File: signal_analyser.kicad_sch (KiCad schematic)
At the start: 0 parts

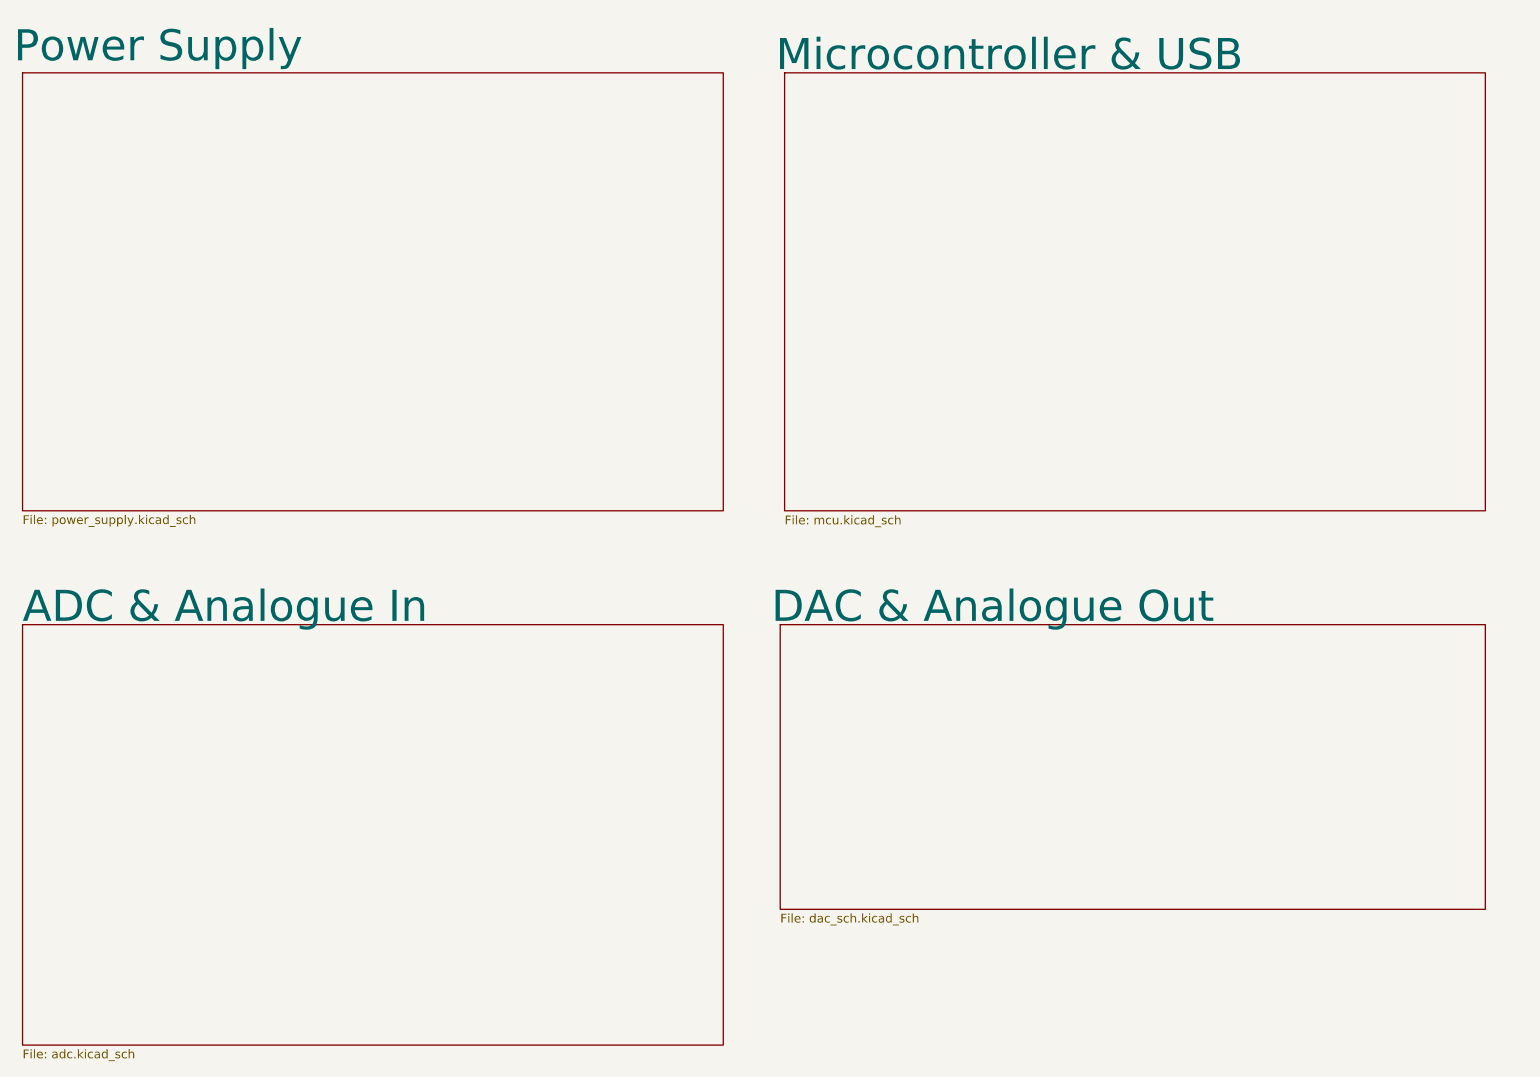
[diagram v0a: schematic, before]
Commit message: ERC valid.
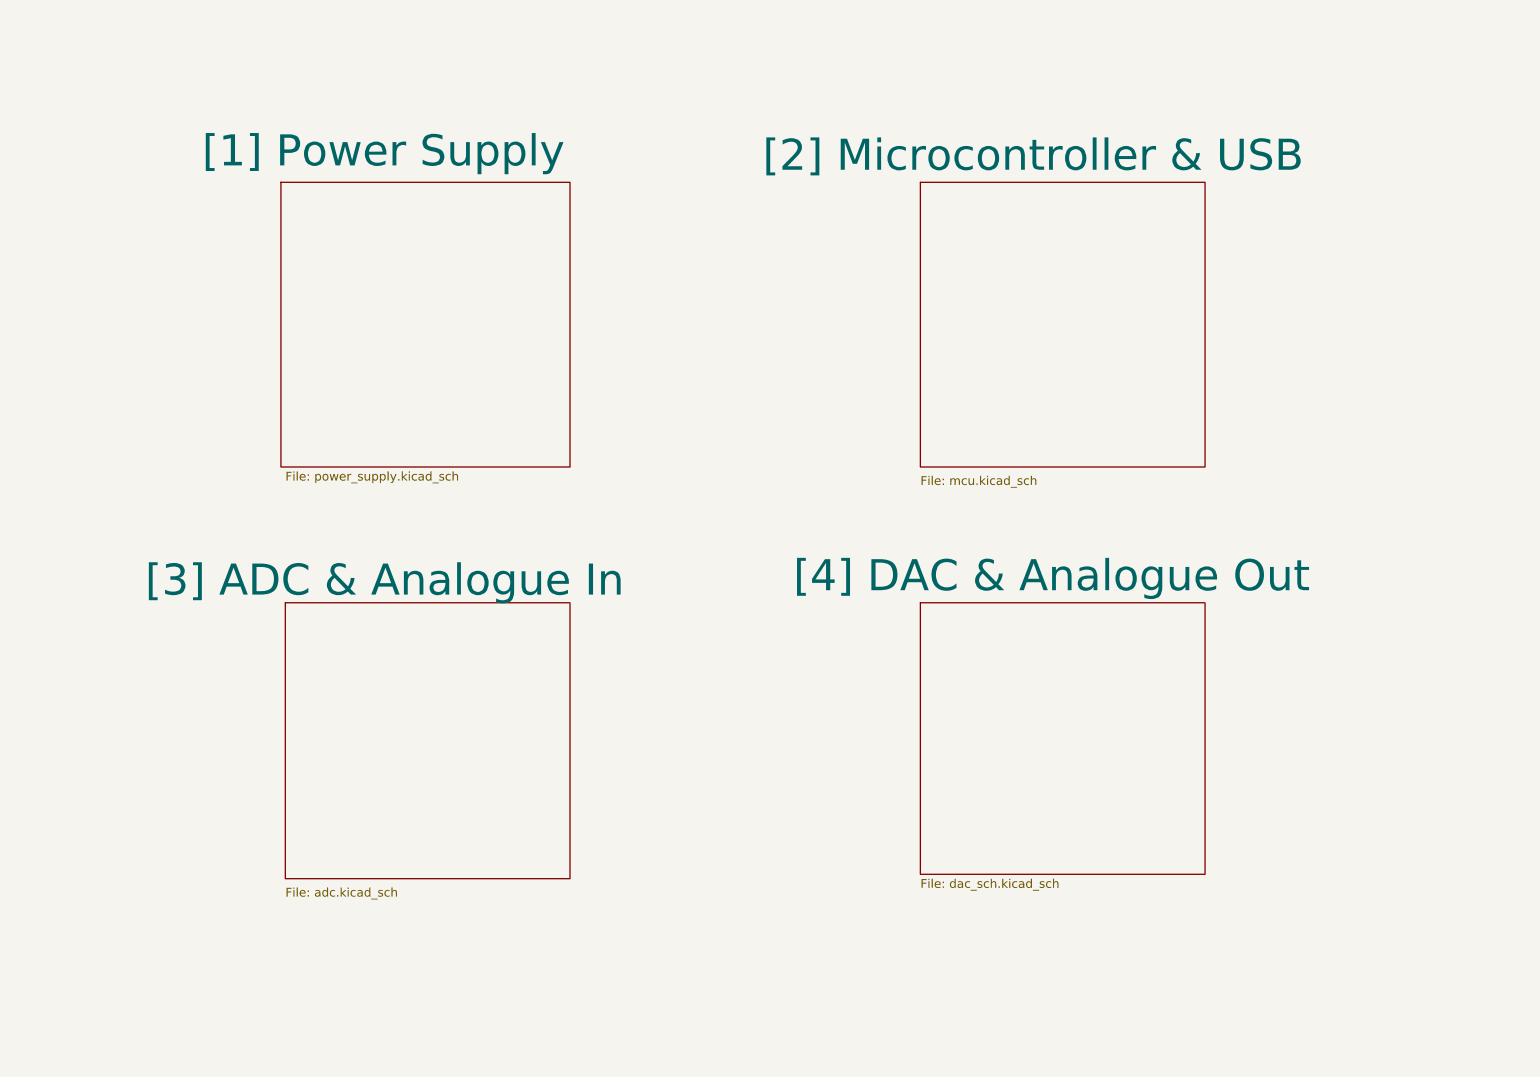
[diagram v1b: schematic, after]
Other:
- sheet ADC & Analogue In renamed [3] ADC & Analogue In
- sheet DAC & Analogue Out renamed [4] DAC & Analogue Out
- sheet Microcontroller & USB renamed [2] Microcontroller & USB
- sheet Power Supply renamed [1] Power Supply
